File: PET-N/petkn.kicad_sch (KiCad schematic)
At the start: 82 parts, among them J1 Extended_PET_keyboard_connect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, J2 Conn_02x03_Odd_Even, J3 LINK3, J5 SPACE1, J6 SPACE2, J67 LINK67, SW1 KP "=", SW10 KP "0", SW11 R SHIFT, SW12 ">", SW14 "]", SW15 "@", SW16 L SHIFT, SW17 KP "+", SW18 KP "2", SW2 KP ".", SW20 "?", SW21 ",", SW22 "N", SW23 "V", SW24 "X", SW25 KP "3", SW26 KP "1", SW27 RETURN, SW28 ";", SW29 "M", SW3 NC ($10), SW30 "B", SW31 "C", SW32 "Z", SW320 S LOCK, SW33 KP "*", SW34 KP "5", SW36 ":", SW37 "K", SW38 "H", SW39 "F", SW4 STOP, SW40 "S", SW41 KP "6", SW42 KP "4", SW44 "L", SW45 "J", SW46 "G", SW47 "D", SW48 "A", SW49 KP "/", SW5 "<", SW50 KP "8", SW52 "P", SW53 "I", SW54 "Y", SW55 "R", SW56 "W", SW57 KP "9", SW58 KP "7", SW59 U ARROW, SW6 SPACE, SW60 "O", SW61 "U", SW62 "T", SW63 "E", SW64 "Q", SW65 INS/DEL, SW66 UP/DOWN, SW67 NC ($0A), SW68 ")", SW69 "\", SW7 "[", SW70 "'", SW71 "$", SW72 QUOTE, SW73 LEFT/RIGHT, SW74 CLR/HOME, SW75 B ARROW, SW76 "(", SW77 "&", SW78 "%", SW79 "#", SW8 OFF/RVS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

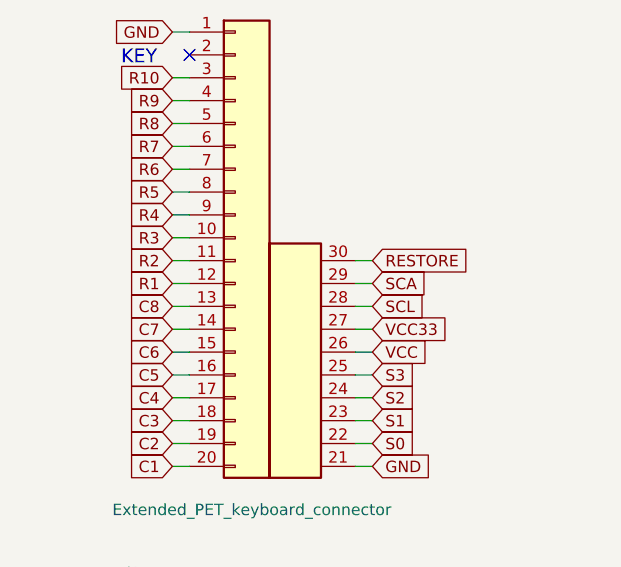
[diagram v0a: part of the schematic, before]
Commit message: PET-N r3
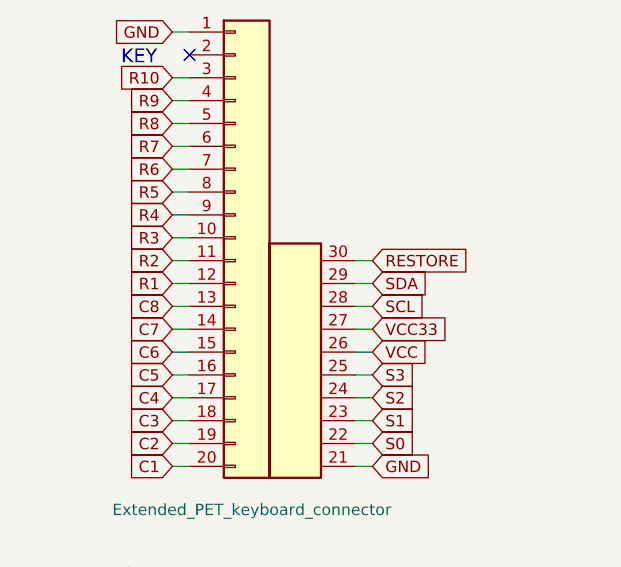
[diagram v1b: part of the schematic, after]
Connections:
- net SCA renamed SDA
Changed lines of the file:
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@@
 		)
 	)
-	(global_label "SCA"
+	(global_label "SDA"
 		(shape input)
 		(at 271.78 54.61 0)

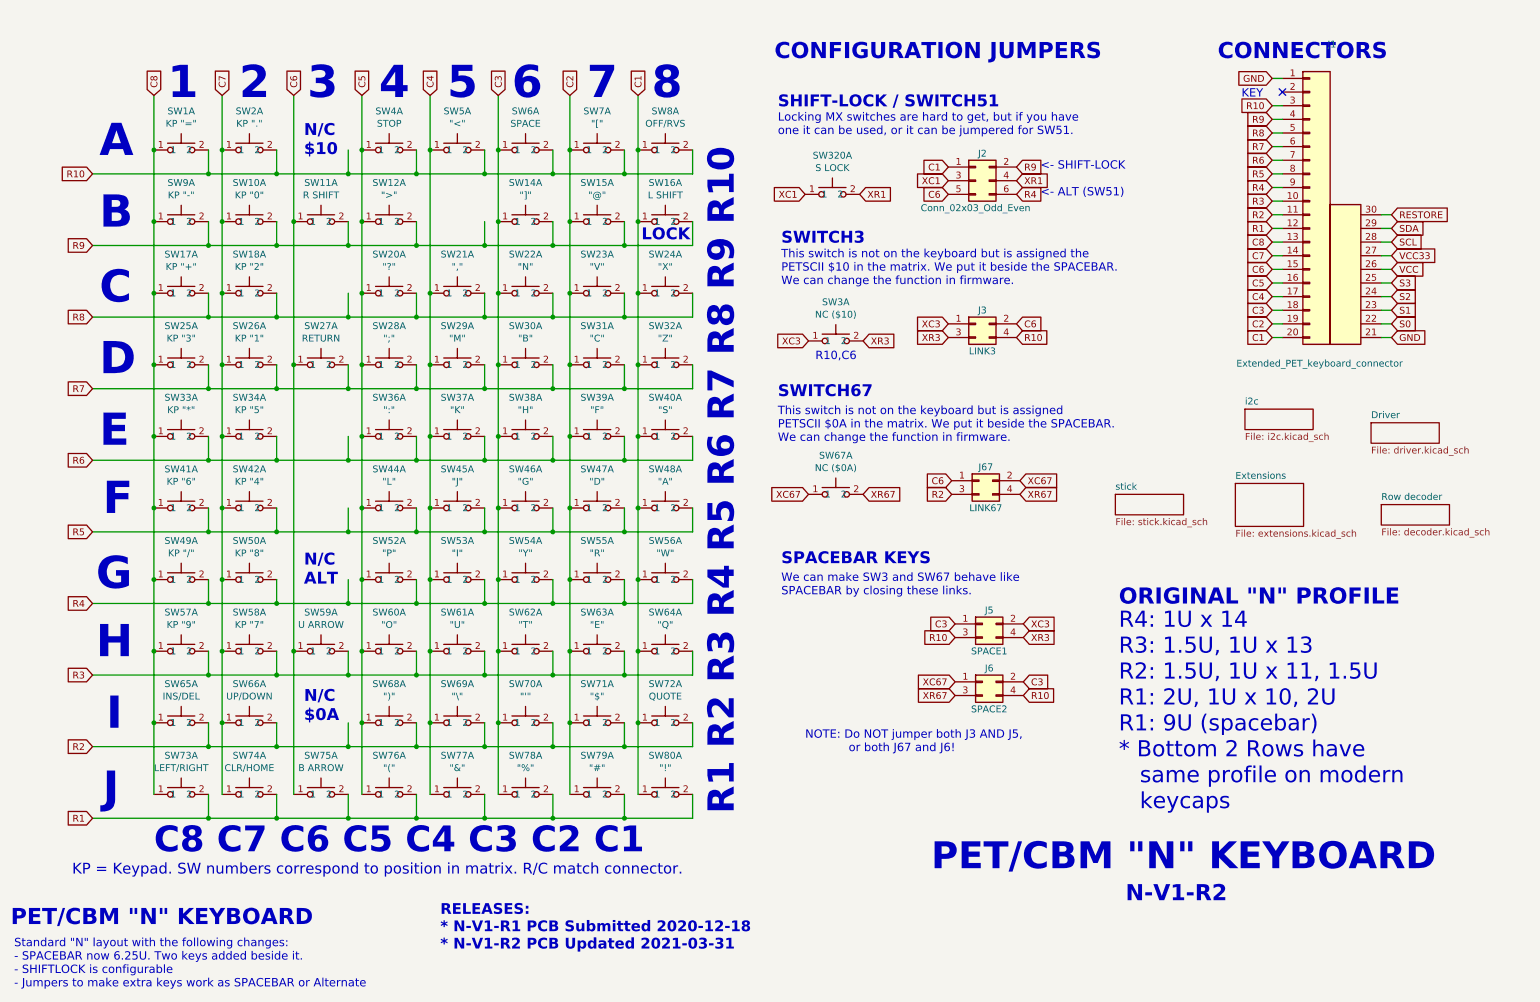
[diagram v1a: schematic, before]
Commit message: new schematics version mainly complete
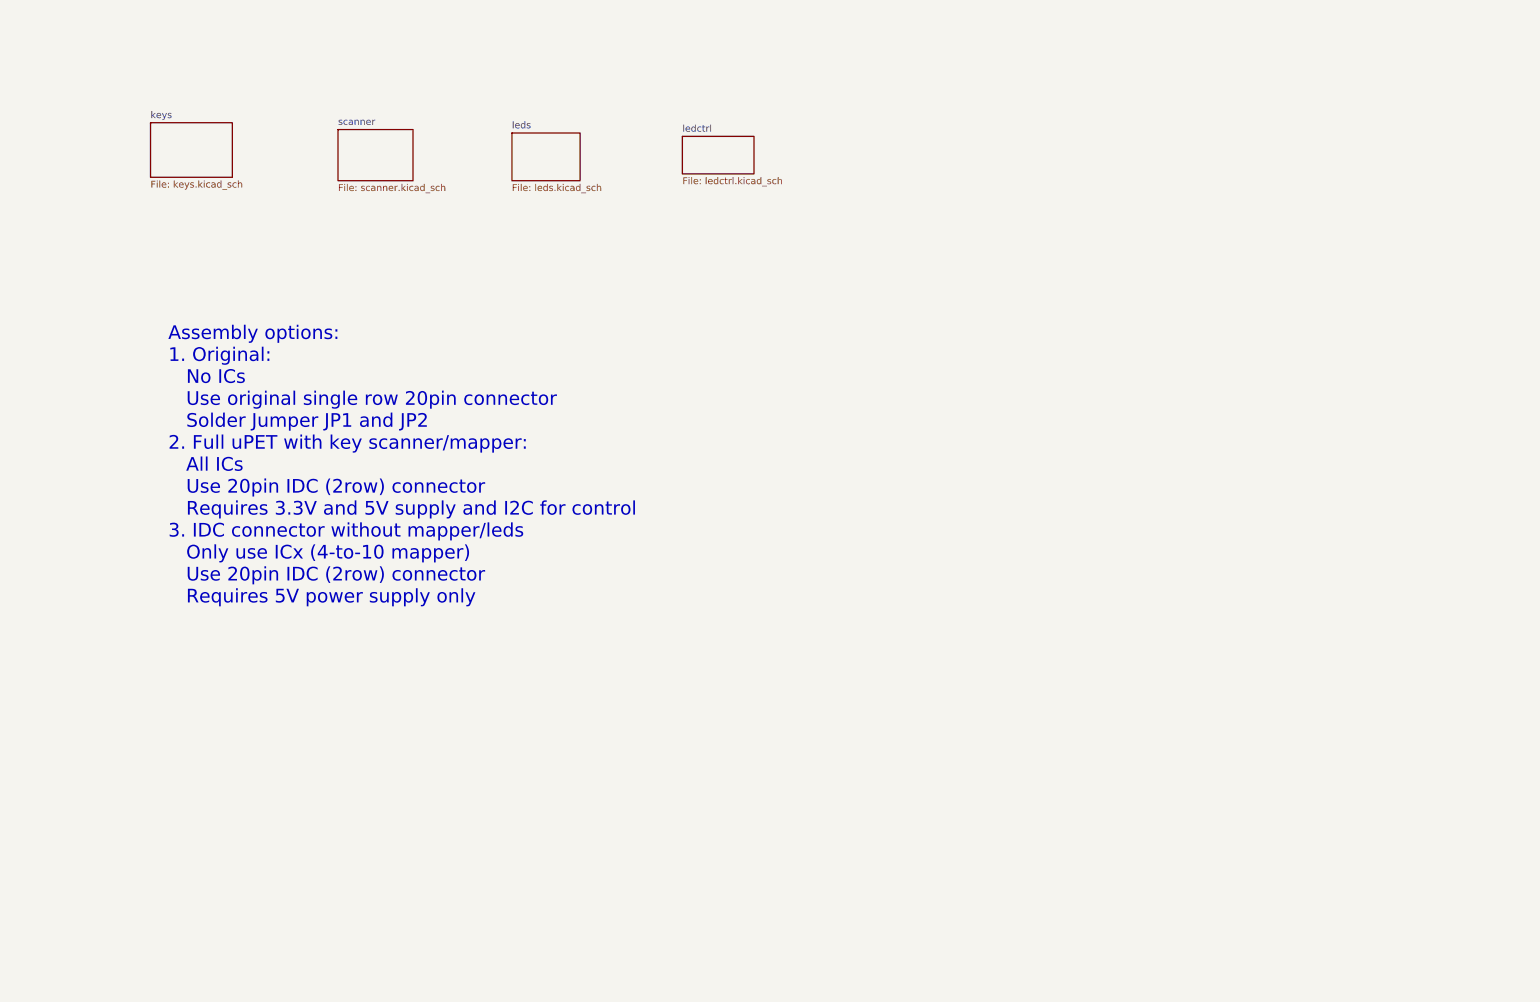
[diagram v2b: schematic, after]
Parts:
- removed J1: Extended_PET_keyboard_connector, petkn:PET_Extended_Keyboard_Connector, symbol petkn:Extended_PET_keyboard_connector
- removed J2: Conn_02x03_Odd_Even, Connector_PinHeader_2.54mm:PinHeader_2x03_P2.54mm_Vertical, symbol Connector_Generic:Conn_02x03_Odd_Even
- removed J3: LINK3, Connector_PinHeader_2.54mm:PinHeader_2x02_P2.54mm_Vertical, symbol Connector_Generic:Conn_02x02_Odd_Even
- removed J5: SPACE1, Connector_PinHeader_2.54mm:PinHeader_2x02_P2.54mm_Vertical, symbol Connector_Generic:Conn_02x02_Odd_Even
- removed J6: SPACE2, Connector_PinHeader_2.54mm:PinHeader_2x02_P2.54mm_Vertical, symbol Connector_Generic:Conn_02x02_Odd_Even
- removed J67: LINK67, Connector_PinHeader_2.54mm:PinHeader_2x02_P2.54mm_Vertical, symbol Connector_Generic:Conn_02x02_Odd_Even
- removed SW1: KP "=", petkn:SW_Cherry_MX_1.00u_PCB_with_LED, symbol petkn:MX Key with LED Unit
- removed SW10: KP "0", petkn:SW_Cherry_MX_1.00u_PCB_with_LED, symbol petkn:MX Key with LED Unit
- removed SW11: R SHIFT, petkn:SW_Cherry_MX_2.00u_PCB_with_LED, symbol petkn:MX Key with LED Unit
- removed SW12: ">", petkn:SW_Cherry_MX_1.00u_PCB_with_LED, symbol petkn:MX Key with LED Unit
- removed SW14: "]", petkn:SW_Cherry_MX_1.00u_PCB_with_LED, symbol petkn:MX Key with LED Unit
- removed SW15: "@", petkn:SW_Cherry_MX_1.00u_PCB_with_LED, symbol petkn:MX Key with LED Unit
- removed SW16: L SHIFT, petkn:SW_Cherry_MX_2.00u_PCB_with_LED, symbol petkn:MX Key with LED Unit
- removed SW17: KP "+", petkn:SW_Cherry_MX_1.00u_PCB_with_LED, symbol petkn:MX Key with LED Unit
- removed SW18: KP "2", petkn:SW_Cherry_MX_1.00u_PCB_with_LED, symbol petkn:MX Key with LED Unit
- removed SW2: KP ".", petkn:SW_Cherry_MX_1.00u_PCB_with_LED, symbol petkn:MX Key with LED Unit
- removed SW20: "?", petkn:SW_Cherry_MX_1.00u_PCB_with_LED, symbol petkn:MX Key with LED Unit
- removed SW21: ",", petkn:SW_Cherry_MX_1.00u_PCB_with_LED, symbol petkn:MX Key with LED Unit
- removed SW22: "N", petkn:SW_Cherry_MX_1.00u_PCB_with_LED, symbol petkn:MX Key with LED Unit
- removed SW23: "V", petkn:SW_Cherry_MX_1.00u_PCB_with_LED, symbol petkn:MX Key with LED Unit
- removed SW24: "X", petkn:SW_Cherry_MX_1.00u_PCB_with_LED, symbol petkn:MX Key with LED Unit
- removed SW25: KP "3", petkn:SW_Cherry_MX_1.00u_PCB_with_LED, symbol petkn:MX Key with LED Unit
- removed SW26: KP "1", petkn:SW_Cherry_MX_1.00u_PCB_with_LED, symbol petkn:MX Key with LED Unit
- removed SW27: RETURN, petkn:SW_Cherry_MX_1.50u_PCB_with_LED, symbol petkn:MX Key with LED Unit
- removed SW28: ";", petkn:SW_Cherry_MX_1.00u_PCB_with_LED, symbol petkn:MX Key with LED Unit
- removed SW29: "M", petkn:SW_Cherry_MX_1.00u_PCB_with_LED, symbol petkn:MX Key with LED Unit
- removed SW3: NC ($10), petkn:SW_Cherry_MX_1.25u_PCB_with_LED, symbol petkn:MX Key with LED Unit
- removed SW30: "B", petkn:SW_Cherry_MX_1.00u_PCB_with_LED, symbol petkn:MX Key with LED Unit
- removed SW31: "C", petkn:SW_Cherry_MX_1.00u_PCB_with_LED, symbol petkn:MX Key with LED Unit
- removed SW32: "Z", petkn:SW_Cherry_MX_1.00u_PCB_with_LED, symbol petkn:MX Key with LED Unit
- removed SW320: S LOCK, petkn:SW_Cherry_MX_1.50u_PCB_with_LED, symbol petkn:MX Key with LED Unit
- removed SW33: KP "*", petkn:SW_Cherry_MX_1.00u_PCB_with_LED, symbol petkn:MX Key with LED Unit
- removed SW34: KP "5", petkn:SW_Cherry_MX_1.00u_PCB_with_LED, symbol petkn:MX Key with LED Unit
- removed SW36: ":", petkn:SW_Cherry_MX_1.00u_PCB_with_LED, symbol petkn:MX Key with LED Unit
- removed SW37: "K", petkn:SW_Cherry_MX_1.00u_PCB_with_LED, symbol petkn:MX Key with LED Unit
- removed SW38: "H", petkn:SW_Cherry_MX_1.00u_PCB_with_LED, symbol petkn:MX Key with LED Unit
- removed SW39: "F", petkn:SW_Cherry_MX_1.00u_PCB_with_LED, symbol petkn:MX Key with LED Unit
- removed SW4: STOP, petkn:SW_Cherry_MX_1.00u_PCB_with_LED, symbol petkn:MX Key with LED Unit
- removed SW40: "S", petkn:SW_Cherry_MX_1.00u_PCB_with_LED, symbol petkn:MX Key with LED Unit
- removed SW41: KP "6", petkn:SW_Cherry_MX_1.00u_PCB_with_LED, symbol petkn:MX Key with LED Unit
- removed SW42: KP "4", petkn:SW_Cherry_MX_1.00u_PCB_with_LED, symbol petkn:MX Key with LED Unit
- removed SW44: "L", petkn:SW_Cherry_MX_1.00u_PCB_with_LED, symbol petkn:MX Key with LED Unit
- removed SW45: "J", petkn:SW_Cherry_MX_1.00u_PCB_with_LED, symbol petkn:MX Key with LED Unit
- removed SW46: "G", petkn:SW_Cherry_MX_1.00u_PCB_with_LED, symbol petkn:MX Key with LED Unit
- removed SW47: "D", petkn:SW_Cherry_MX_1.00u_PCB_with_LED, symbol petkn:MX Key with LED Unit
- removed SW48: "A", petkn:SW_Cherry_MX_1.00u_PCB_with_LED, symbol petkn:MX Key with LED Unit
- removed SW49: KP "/", petkn:SW_Cherry_MX_1.00u_PCB_with_LED, symbol petkn:MX Key with LED Unit
- removed SW5: "<", petkn:SW_Cherry_MX_1.00u_PCB_with_LED, symbol petkn:MX Key with LED Unit
- removed SW50: KP "8", petkn:SW_Cherry_MX_1.00u_PCB_with_LED, symbol petkn:MX Key with LED Unit
- removed SW52: "P", petkn:SW_Cherry_MX_1.00u_PCB_with_LED, symbol petkn:MX Key with LED Unit
- removed SW53: "I", petkn:SW_Cherry_MX_1.00u_PCB_with_LED, symbol petkn:MX Key with LED Unit
- removed SW54: "Y", petkn:SW_Cherry_MX_1.00u_PCB_with_LED, symbol petkn:MX Key with LED Unit
- removed SW55: "R", petkn:SW_Cherry_MX_1.00u_PCB_with_LED, symbol petkn:MX Key with LED Unit
- removed SW56: "W", petkn:SW_Cherry_MX_1.00u_PCB_with_LED, symbol petkn:MX Key with LED Unit
- removed SW57: KP "9", petkn:SW_Cherry_MX_1.00u_PCB_with_LED, symbol petkn:MX Key with LED Unit
- removed SW58: KP "7", petkn:SW_Cherry_MX_1.00u_PCB_with_LED, symbol petkn:MX Key with LED Unit
- removed SW59: U ARROW, petkn:SW_Cherry_MX_1.00u_PCB_with_LED, symbol petkn:MX Key with LED Unit
- removed SW6: SPACE, petkn:SW_Cherry_MX_6.25u_PCB_with_LED, symbol petkn:MX Key with LED Unit
- removed SW60: "O", petkn:SW_Cherry_MX_1.00u_PCB_with_LED, symbol petkn:MX Key with LED Unit
- removed SW61: "U", petkn:SW_Cherry_MX_1.00u_PCB_with_LED, symbol petkn:MX Key with LED Unit
- removed SW62: "T", petkn:SW_Cherry_MX_1.00u_PCB_with_LED, symbol petkn:MX Key with LED Unit
- removed SW63: "E", petkn:SW_Cherry_MX_1.00u_PCB_with_LED, symbol petkn:MX Key with LED Unit
- removed SW64: "Q", petkn:SW_Cherry_MX_1.00u_PCB_with_LED, symbol petkn:MX Key with LED Unit
- removed SW65: INS/DEL, petkn:SW_Cherry_MX_1.00u_PCB_with_LED, symbol petkn:MX Key with LED Unit
- removed SW66: UP/DOWN, petkn:SW_Cherry_MX_1.00u_PCB_with_LED, symbol petkn:MX Key with LED Unit
- removed SW67: NC ($0A), petkn:SW_Cherry_MX_1.50u_PCB_with_LED, symbol petkn:MX Key with LED Unit
- removed SW68: ")", petkn:SW_Cherry_MX_1.00u_PCB_with_LED, symbol petkn:MX Key with LED Unit
- removed SW69: "\", petkn:SW_Cherry_MX_1.00u_PCB_with_LED, symbol petkn:MX Key with LED Unit
- removed SW7: "[", petkn:SW_Cherry_MX_1.00u_PCB_with_LED, symbol petkn:MX Key with LED Unit
- removed SW70: "'", petkn:SW_Cherry_MX_1.00u_PCB_with_LED, symbol petkn:MX Key with LED Unit
- removed SW71: "$", petkn:SW_Cherry_MX_1.00u_PCB_with_LED, symbol petkn:MX Key with LED Unit
- removed SW72: QUOTE, petkn:SW_Cherry_MX_1.00u_PCB_with_LED, symbol petkn:MX Key with LED Unit
- removed SW73: LEFT/RIGHT, petkn:SW_Cherry_MX_1.00u_PCB_with_LED, symbol petkn:MX Key with LED Unit
- removed SW74: CLR/HOME, petkn:SW_Cherry_MX_1.00u_PCB_with_LED, symbol petkn:MX Key with LED Unit
- removed SW75: B ARROW, petkn:SW_Cherry_MX_1.00u_PCB_with_LED, symbol petkn:MX Key with LED Unit
- removed SW76: "(", petkn:SW_Cherry_MX_1.00u_PCB_with_LED, symbol petkn:MX Key with LED Unit
- removed SW77: "&", petkn:SW_Cherry_MX_1.00u_PCB_with_LED, symbol petkn:MX Key with LED Unit
- removed SW78: "%", petkn:SW_Cherry_MX_1.00u_PCB_with_LED, symbol petkn:MX Key with LED Unit
- removed SW79: "#", petkn:SW_Cherry_MX_1.00u_PCB_with_LED, symbol petkn:MX Key with LED Unit
- removed SW8: OFF/RVS, petkn:SW_Cherry_MX_1.50u_PCB_with_LED, symbol petkn:MX Key with LED Unit
- removed SW80: "!", petkn:SW_Cherry_MX_1.00u_PCB_with_LED, symbol petkn:MX Key with LED Unit
- removed SW9: KP "-", petkn:SW_Cherry_MX_1.00u_PCB_with_LED, symbol petkn:MX Key with LED Unit
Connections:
- no-connect marks 1 -> 0
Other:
- removed sheet Driver
- removed sheet Extensions
- removed sheet Row decoder
- removed sheet i2c
- removed sheet stick
- added sheet keys (keys.kicad_sch)
- added sheet ledctrl (ledctrl.kicad_sch)
- added sheet leds (leds.kicad_sch)
- added sheet scanner (scanner.kicad_sch)
- note added: "Assembly options: 1. Original: No ICs Use original single row 20pin connector Solder Jumper JP1 and JP2 2. Full uPET with key scanner/mapper: All ICs Use 20pin IDC (2row) connector Requires 3.3V and 5V supply and I2C for control 3. IDC connector without mapper/leds Only use ICx (4-to-10 mapper) Use 20pin IDC (2row) connector Requires 5V power supply only"
- note removed: "1"
- note removed: "2"
- note removed: "3"
- note removed: "4"
- note removed: "5"
- note removed: "6"
- note removed: "7"
- note removed: "8"
- note removed: "<- SHIFT-LOCK <- ALT (SW51)"
- note removed: "A"
- note removed: "B"
- note removed: "C"
- note removed: "C8 C7 C6 C5 C4 C3 C2 C1"
- note removed: "CONFIGURATION JUMPERS"
- note removed: "CONNECTORS"
- note removed: "D"
- note removed: "E"
- note removed: "F"
- note removed: "G"
- note removed: "H"
- note removed: "I"
- note removed: "J"
- note removed: "KEY"
- note removed: "KP = Keypad. SW numbers correspond to position in matrix. R/C match connector."
- note removed: "LOCK"
- note removed: "Locking MX switches are hard to get, but if you have one it can be used, or it can be jumpered for SW51."
- note removed: "N-V1-R2"
- note removed: "N/C $0A"
- note removed: "N/C $10"
- note removed: "N/C ALT"
- note removed: "NOTE: Do NOT jumper both J3 AND J5, or both J67 and J6!"
- note removed: "ORIGINAL "N" PROFILE"
- note removed: "PET/CBM "N" KEYBOARD"
- note removed: "R1 R2 R3 R4 R5 R6 R7 R8 R9 R10"
- note removed: "R10,C6"
- note removed: "R4: 1U x 14 R3: 1.5U, 1U x 13 R2: 1.5U, 1U x 11, 1.5U R1: 2U, 1U x 10, 2U R1: 9U (spacebar) * Bottom 2 Rows have same profile on modern keycaps"
- note removed: "RELEASES: * N-V1-R1 PCB Submitted 2020-12-18 * N-V1-R2 PCB Updated 2021-03-31"
- note removed: "SHIFT-LOCK / SWITCH51"
- note removed: "SPACEBAR KEYS"
- note removed: "SWITCH3"
- note removed: "SWITCH67"
- note removed: "Standard "N" layout with the following changes: - SPACEBAR now 6.25U. Two keys added beside it. - SHIFTLOCK is configurable - Jumpers to make extra keys work as SPACEBAR or Alternate"
- note removed: "This switch is not on the keyboard but is assigned PETSCII $0A in the matrix. We put it beside the SPACEBAR. We can change the function in firmware."
- note removed: "This switch is not on the keyboard but is assigned the PETSCII $10 in the matrix. We put it beside the SPACEBAR. We can change the function in firmware."
- note removed: "We can make SW3 and SW67 behave like SPACEBAR by closing these links."
